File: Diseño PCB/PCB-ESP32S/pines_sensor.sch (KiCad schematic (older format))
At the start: 1 part, among them U2 pines_sensor

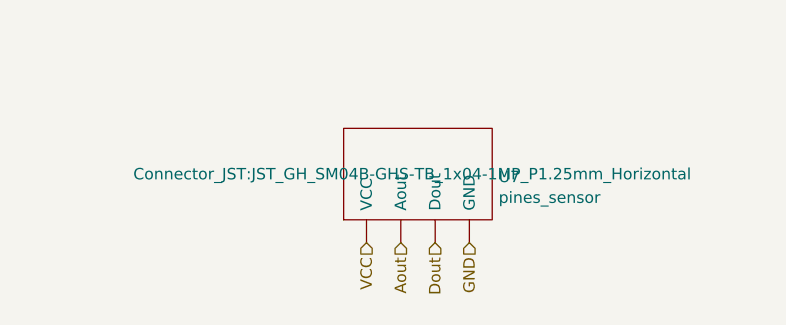
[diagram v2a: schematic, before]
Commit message: separacion
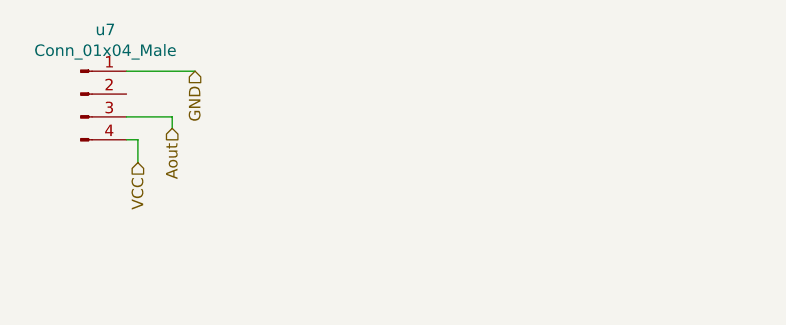
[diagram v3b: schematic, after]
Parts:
- removed U2: pines_sensor, Connector_JST:JST_GH_SM04B-GHS-TB_1x04-1MP_P1.25mm_Horizontal, symbol PCB-ESP32S-rescue:pines_sensor-pines_yl100&mq135-PCB-ESP32S-rescue
- added u7: Conn_01x04_Male, Connector_JST:JST_GH_BM04B-GHS-TBT_1x04-1MP_P1.25mm_Vertical, symbol Connector:Conn_01x04_Male
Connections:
- net Aout: now also u7.3 (Pin_3)
- net GND: now also u7.1 (Pin_1)
- net VCC: now also u7.4 (Pin_4)
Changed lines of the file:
@@
 $Descr A4 11693 8268
 encoding utf-8
-Sheet 7 7
+Sheet 4 6
 Title ""
 Date ""
@@
 Comment4 ""
 $EndDescr
+Text HLabel 1850 2300 3    50   Input ~ 0
+VCC
+Text HLabel 2000 2150 3    50   Input ~ 0
+Aout
+Text HLabel 2100 1900 3    50   Input ~ 0
+GND
 $Comp
-L PCB-ESP32S-rescue:pines_sensor-pines_yl100&mq135-PCB-ESP32S-rescue U2
-U 1 1 619FDFBF
-P 3050 2350
-AR Path="/619FC5E1/619FDFBF" Ref="U2"  Part="1"
-AR Path="/61A90AD5/619FDFBF" Ref="U7"  Part="1"
-F 0 "U7" H 3428 2338 50  0000 L CNN
-F 1 "pines_sensor" H 3428 2247 50  0000 L CNN
-F 2 "Connector_JST:JST_GH_SM04B-GHS-TB_1x04-1MP_P1.25mm_Horizontal" H 3050 2350 50  0000 C CNN
-F 3 "" H 3050 2350 50  0001 C CNN
-	1    3050 2350
+L Connector:Conn_01x04_Male u7
+U 1 1 61E262EF
+P 1600 2000
+F 0 "u7" H 1708 2281 50  0000 C CNN
+F 1 "Conn_01x04_Male" H 1708 2190 50  0000 C CNN
+F 2 "Connector_JST:JST_GH_BM04B-GHS-TBT_1x04-1MP_P1.25mm_Vertical" H 1600 2000 50  0001 C CNN
+F 3 "~" H 1600 2000 50  0001 C CNN
+	1    1600 2000
 	1    0    0    -1
 $EndComp
-Text HLabel 2850 2650 3    50   Input ~ 0
-VCC
-Text HLabel 3000 2650 3    50   Input ~ 0
-Aout
-Text HLabel 3150 2650 3    50   Input ~ 0
-Dout
-Text HLabel 3300 2650 3    50   Input ~ 0
-GND
+Wire Wire Line
+	1800 1900 2100 1900
+Wire Wire Line
+	1800 2100 2000 2100
+Wire Wire Line
+	2000 2100 2000 2150
+Wire Wire Line
+	1800 2200 1850 2200
+Wire Wire Line
+	1850 2200 1850 2300
 $EndSCHEMATC
